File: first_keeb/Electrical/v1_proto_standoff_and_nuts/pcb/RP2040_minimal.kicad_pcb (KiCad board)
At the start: 4 copper layers, 67.1 x 66.8 mm, 68 parts, among them P1 USB-TYPE-C-016, Q1 SN74LV1T34DBV, SW1 SKRKAHE020, SW2 BUTT0, SW3 BUTT1, U1 NCP1117-3.3_SOT223, U2 MCP1525-TT, U3 PRTR5V0U2X, U4 MCP6004, U5 STM32F401RCTx, Y1 16MHz

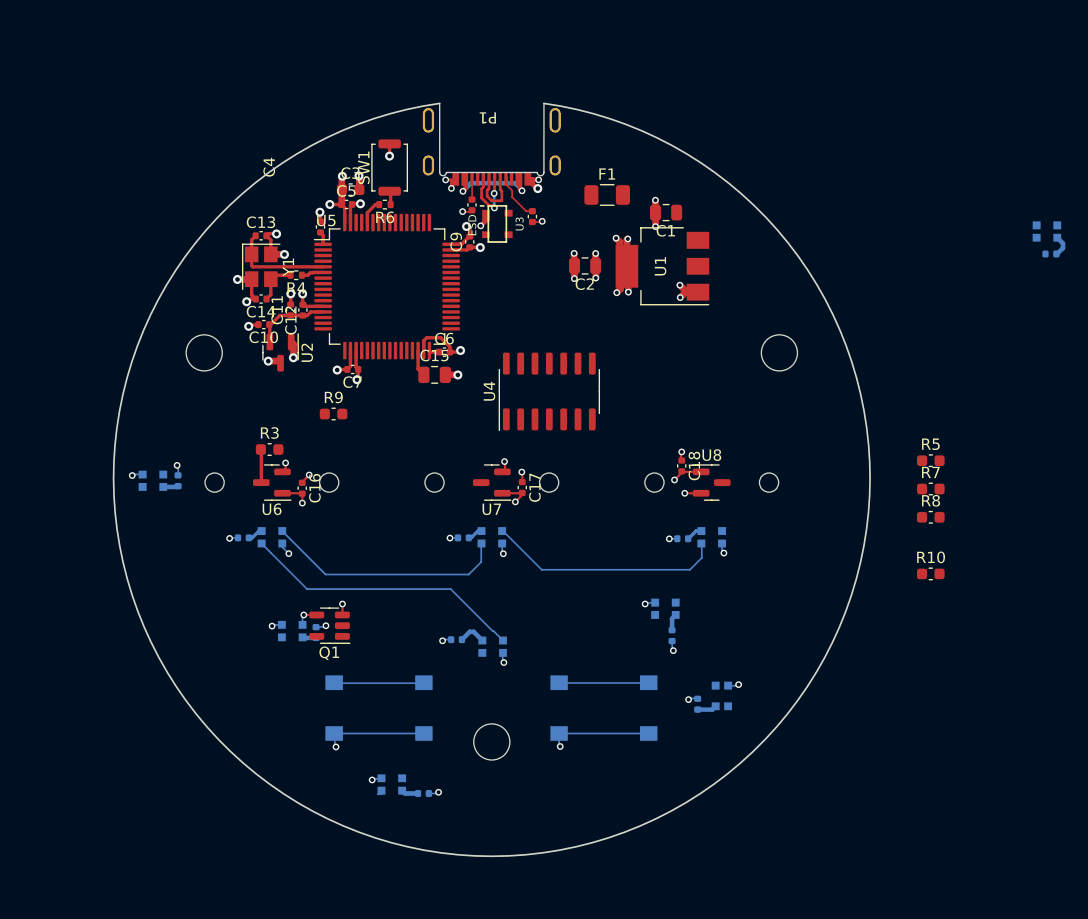
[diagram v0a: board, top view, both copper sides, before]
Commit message: stm32 pcb almost done
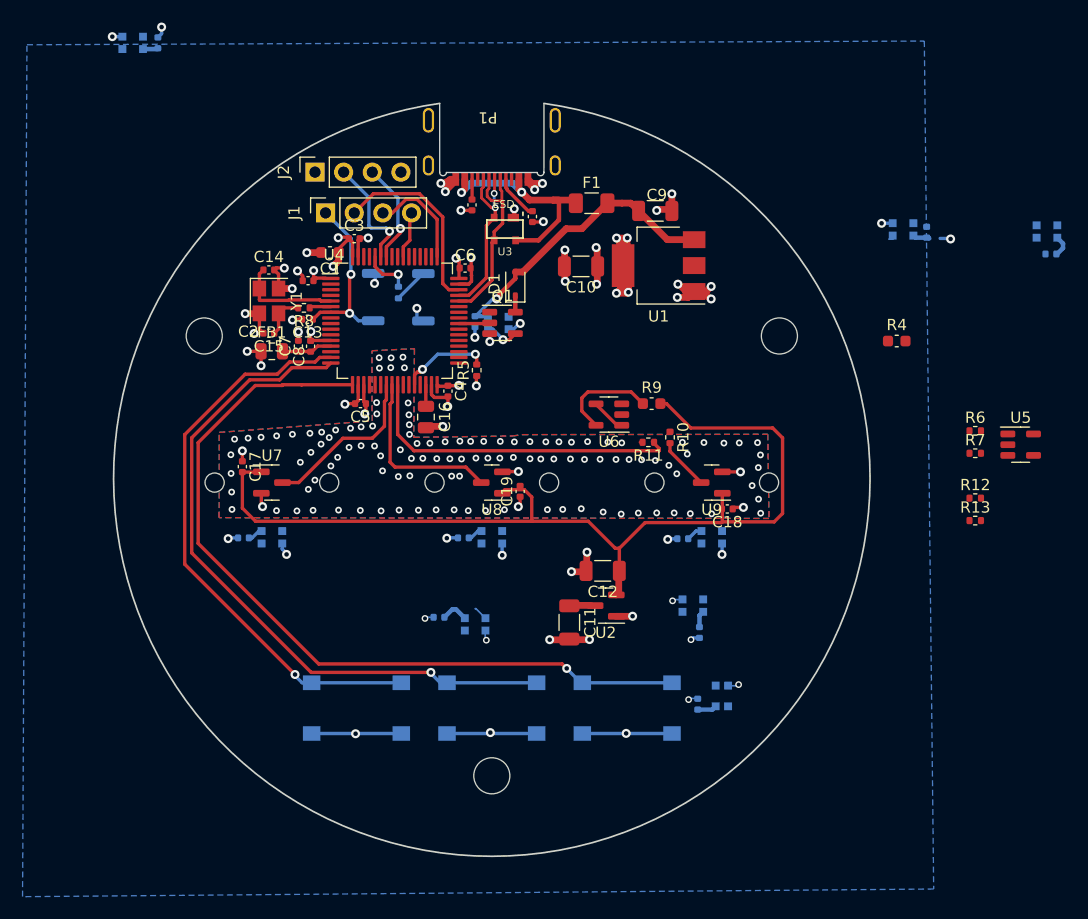
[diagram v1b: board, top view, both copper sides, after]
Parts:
- removed the C1 at (115.5, 76.1)
- removed the C2 at (108.3, 80.8)
- removed the R3 at (80.3, 97.1)
- removed the R8 at (138.9, 103.1)
- removed the U4 at (105.1, 91.9)
- added C11: 10u, Capacitor_SMD:C_1206_3216Metric, F.Cu at (106.9, 112.4)
- added C12: 10u, Capacitor_SMD:C_1206_3216Metric, F.Cu at (109.8, 107.8)
- added C13: 100n, Capacitor_SMD:C_0402_1005Metric, F.Cu at (83.7, 85.5)
- added C6: 100n, Capacitor_SMD:C_0402_1005Metric, F.Cu at (97.6, 81.0)
- added D1: 1N4148WS, Diode_SMD:D_SOD-323, F.Cu at (102.1, 82.4)
- added FB1: GZ2012D601TF, Capacitor_SMD:C_0805_2012Metric, F.Cu at (80.5, 88.4)
- added J1: Conn_01x04_Socket, Connector_PinSocket_2.54mm:PinSocket_1x04_P2.54mm_Vertical, F.Cu at (85.3, 76.1)
- added J2: Conn_01x04_Socket, Connector_PinSocket_2.54mm:PinSocket_1x04_P2.54mm_Vertical, F.Cu at (84.3, 72.5)
- added R11: DNP, Resistor_SMD:R_0402_1005Metric, F.Cu at (113.9, 96.4)
- added R12: 0, Resistor_SMD:R_0402_1005Metric, F.Cu at (142.9, 101.4)
- added R13: 0, Resistor_SMD:R_0402_1005Metric, F.Cu at (142.9, 103.4)
- added R4: DNP, Capacitor_SMD:C_0603_1608Metric, F.Cu at (135.9, 87.5)
- added R6: DNP, Resistor_SMD:R_0402_1005Metric, F.Cu at (142.9, 95.4)
- added SW2: SKRKAHE020, Button_Switch_SMD:SW_Push_SPST_NO_Alps_SKRK, B.Cu at (89.5, 83.5)
- added SW4: BUTT3, Button_Switch_SMD:SW_Push_1P1T_NO_6x6mm_H9.5mm, B.Cu at (112.0, 120.0)
- added U5: MCP6001-OT, Package_TO_SOT_SMD:SOT-23-5, F.Cu at (146.9, 96.6)
- added U6: MCP6001-OT, Package_TO_SOT_SMD:SOT-23-5, F.Cu at (110.4, 94.0)
- C10: value 1u -> 10u; footprint Capacitor_SMD:C_0402_1005Metric -> Capacitor_SMD:C_1206_3216Metric
- C9: value 100n -> 10u; footprint Capacitor_SMD:C_0402_1005Metric -> Capacitor_SMD:C_1206_3216Metric
- R10, R7: value 0 -> DNP; footprint Capacitor_SMD:C_0603_1608Metric -> Resistor_SMD:R_0402_1005Metric
- R3: renamed from R6; moved to B.Cu
- R5: value 0 -> 10k; footprint Capacitor_SMD:C_0603_1608Metric -> Resistor_SMD:R_0402_1005Metric
- R9: value 0 -> DNP
- SW1: moved to B.Cu
- SW3: renamed from SW2; value BUTT0 -> BUTT1
- SW5: renamed from SW3; value BUTT1 -> BUTT2
- U1: value NCP1117-3.3_SOT223 -> AMS1117-2.5
- U2: value MCP1525-TT -> ME6208A44M3G
- moved D4 66.9 mm to (136.5, 77.5)
- moved C22 66.8 mm to (138.6, 77.8), turned to 90 degrees
- moved R5 41.1 mm to (98.7, 90.0), turned to 90 degrees
- moved C21 38.9 mm to (70.4, 61.0)
- moved D3 38.9 mm to (68.2, 61.0)
- moved U2 36.5 mm to (110.1, 110.9), turned to 180 degrees
- moved D2 32.9 mm to (100.6, 85.8), turned to 180 degrees
- moved C20 31.0 mm to (98.5, 85.7), turned to -90 degrees
- moved Q1 30.9 mm to (101.0, 85.8), turned to 0 degrees
- moved C10 28.6 mm to (107.9, 80.8)
- moved R9 28.2 mm to (114.2, 93.0)
- moved R10 26.1 mm to (115.8, 96.0), turned to -90 degrees
- moved U8 19.5 mm to (100.0, 100.0), turned to 180 degrees
- moved U9 19.5 mm to (119.5, 100.0)
- moved C18 18.3 mm to (120.9, 102.3), turned to 180 degrees
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- renumbered C3 to C1, C13 to C14, C14 to C15, C15 to C16, C16 to C17, C17 to C18, C18 to C19, C4 to C2, C19 to C20, C20 to C21, C21 to C22, C22 to C23, C23 to C24, C24 to C25, C25 to C26, C26 to C27, C27 to C28, C28 to C29, C5 to C3, C6 to C4, C7 to C5, C11 to C7, C12 to C8, D9 to D10, D10 to D11, D1 to D2, D2 to D3, D3 to D4, D4 to D5, D5 to D6, D6 to D7, D7 to D8, D8 to D9, R4 to R8, U5 to U4, U6 to U7, U7 to U9
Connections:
- C1 pad 1: +3V3 -> VDD
- C10 pad 1: ADC_VREF -> VDD
- C17 pad 2: +3V3 -> V_test
- C18 pad 2: +3V3 -> V_test
- C19 pad 2: +3V3 -> V_test
- C2 pad 1: +3V3 -> VDD
- C3 pad 1: +3V3 -> VDD
- C4 pad 1: +3V3 -> VDD
- C5 pad 1: +3V3 -> VDD
- C7 pad 1: ADC_VREF -> VDDA
- C8 pad 1: ADC_VREF -> VDDA
- C9 pad 1: GND -> +5V
- C9 pad 2: +3V3 -> GND
- Q1 pad 2: LED_D_5V -> LED_D
- Q1 pad 5: +5V -> Net-(D1-K)
- R10 pad 1: A_OUT2 -> Net-(U6-+)
- R10 pad 2: ADC_IN2 -> ALT_ADC_3
- R5 pad 1: A_OUT2 -> GND
- R5 pad 2: Net-(U4B-+) -> BOOT1
- R7 pad 1: A_OUT3 -> ADC_IN2
- R9 pad 1: A_OUT1 -> Net-(U6-V+)
- R9 pad 2: ADC_IN1 -> V_test
- SW1 pad 2: +3V3 -> VDD
- SW3 pad 1: unconnected-(SW2-Pad1) -> BUTT0
- SW5 pad 1: unconnected-(SW3-Pad1) -> BUTT1
- U1 pad 2: +3V3 -> VDD
- U2 pad 1: +3V3 -> GND
- U2 pad 2: ADC_VREF -> V_test
- U2 pad 3: GND -> +5V
- U4 pad 1: +3V3 -> VDD
- U4 pad 13: ADC_VREF -> VDDA
- U4 pad 15: unconnected-(U5-PA1-Pad15) -> BUTT0
- U4 pad 16: unconnected-(U5-PA2-Pad16) -> BUTT1
- U4 pad 17: unconnected-(U5-PA3-Pad17) -> BUTT2
- U4 pad 19: +3V3 -> VDD
- U4 pad 22: ALT_ADC_IN1 -> unconnected-(U4-PA6-Pad22)
- U4 pad 23: ALT_ADC_IN2 -> ADC_IN1
- U4 pad 24: ALT_ADC_IN3 -> ADC_IN2
- U4 pad 25: ADC_IN1 -> ADC_IN3
- U4 pad 26: ADC_IN2 -> unconnected-(U4-PB0-Pad26)
- U4 pad 27: ADC_IN3 -> unconnected-(U4-PB1-Pad27)
- U4 pad 28: unconnected-(U5-PB2-Pad28) -> BOOT1
- U4 pad 32: +3V3 -> VDD
- U4 pad 40: unconnected-(U5-PC9-Pad40) -> LED_D
- U4 pad 46: unconnected-(U5-PA13-Pad46) -> SWDIO
- U4 pad 48: +3V3 -> VDD
- U4 pad 49: unconnected-(U5-PA14-Pad49) -> SWCLK
- U4 pad 55: unconnected-(U5-PB3-Pad55) -> SWO
- U4 pad 58: unconnected-(U5-PB6-Pad58) -> USART1_TX
- U4 pad 59: unconnected-(U5-PB7-Pad59) -> USART1_RX
- U4 pad 64: +3V3 -> VDD
- U7 pad 1: +3V3 -> V_test
- U7 pad 3: A_OUT1 -> ADC_IN1
- U8 pad 1: +3V3 -> V_test
- U8 pad 3: A_OUT2 -> ALT_ADC_2
- U9 pad 1: +3V3 -> V_test
- U9 pad 3: A_OUT3 -> ALT_ADC_3
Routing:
- net V_test: track 0.00 -> 86.6 mm
- net BUTT2: track 0.00 -> 71.9 mm, vias 0 -> 1
- net BUTT1: track 0.00 -> 60.9 mm, vias 0 -> 1
- net BUTT0: track 0.00 -> 51.1 mm, vias 0 -> 1
- net VDD: track 0.00 -> 33.2 mm, vias 0 -> 15
- net +3V3: track 32.6 -> 0.00 mm, vias 15 -> 0
- net GND: track 81.6 -> 111.4 mm, vias 55 -> 179
- net ADC_IN3: track 0.00 -> 29.2 mm
- net +5V: track 16.2 -> 43.9 mm, vias 0 -> 1
- net Net-(D5-DOUT): track 25.0 -> 1.26 mm
- net Net-(D6-DOUT): track 21.3 -> 0.00 mm
- net Net-(D7-DOUT): track 20.9 -> 0.00 mm
- net SWDIO: track 0.00 -> 17.0 mm
- net NRST: track 0.00 -> 16.3 mm, vias 0 -> 2
- net ADC_IN2: track 0.00 -> 15.8 mm
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- added copper zone on B.Cu, net GND
- added copper zone on F.Cu, net GND
- added copper zone on In2.Cu, net GND
- added copper zone on B.Cu, net VDD
- removed copper zone on In2.Cu, net +3V3
